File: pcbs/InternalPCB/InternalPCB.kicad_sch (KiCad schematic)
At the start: 17 parts, among them J1 Conn_01x20, J10 694106301002, J11 694106301002, J2 Conn_01x20, J3 Conn_01x04_Pin, J4 Conn_01x04_Pin, J5 Conn_01x02_Pin, J6 Conn_01x04_Pin, J7 Conn_01x03_Pin, J8 Conn_01x05_Pin, J9 Conn_01x05_Pin, SW1 SW_Push, U1 Pico W, U2 Pico, U3 004-0-0013

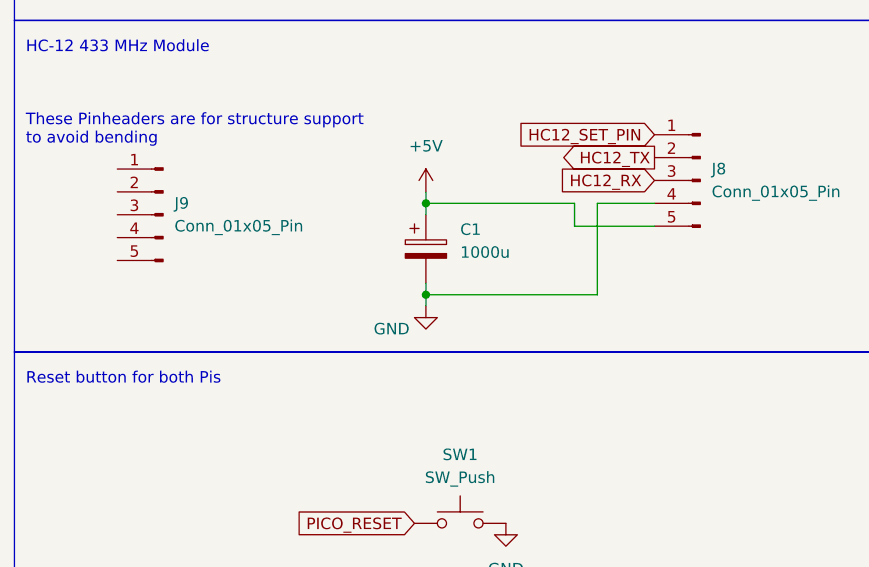
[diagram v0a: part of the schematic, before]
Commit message: Bisschen DRC dies das
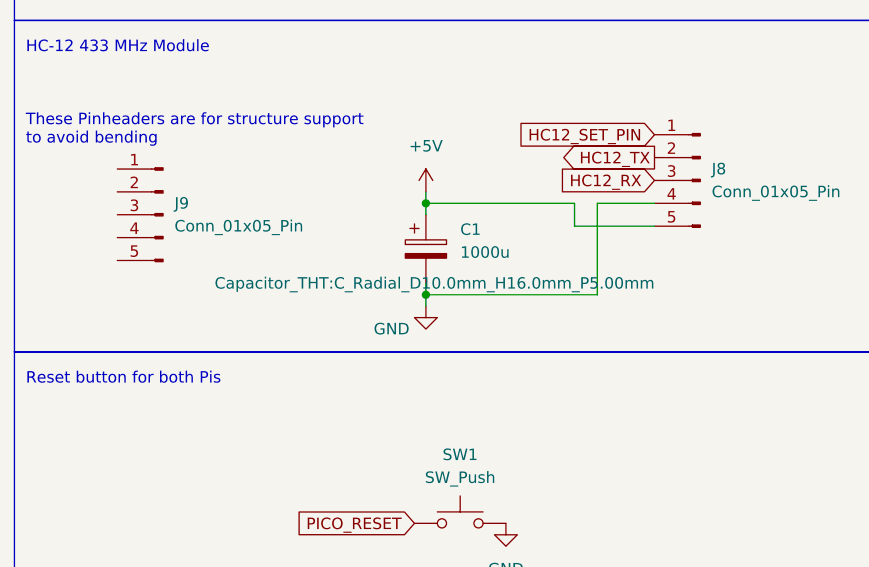
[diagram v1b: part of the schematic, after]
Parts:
- C1: footprint Capacitor_THT:CP_Axial_L46.0mm_D20.0mm_P52.00mm_Horizontal -> Capacitor_THT:C_Radial_D10.0mm_H16.0mm_P5.00mm
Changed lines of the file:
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@@
       (effects (font (size 1.27 1.27)) (justify left))
     )
-    (property "Footprint" "Capacitor_THT:CP_Axial_L46.0mm_D20.0mm_P52.00mm_Horizontal" (at 351.4852 195.58 0)
-      (effects (font (size 1.27 1.27)) hide)
+    (property "Footprint" "Capacitor_THT:C_Radial_D10.0mm_H16.0mm_P5.00mm" (at 351.4852 195.58 0)
+      (effects (font (size 1.27 1.27)))
     )
     (property "Datasheet" "~" (at 350.52 191.77 0)
